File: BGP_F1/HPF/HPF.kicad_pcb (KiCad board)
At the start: 2 copper layers, 30 x 24 mm, 15 parts, among them P1 CONN_01X05, P2 CONN_01X06, U1 MC33178

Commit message: F1 updates to reverse pots
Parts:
- C3: value 39n -> 22n
- R3, R5, R7: value 4.99k -> 4.7k
- R4: value 24.9k -> 24k
- R6: value 49.9k -> 47k
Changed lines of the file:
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@@
       (effects (font (size 0.6 0.6) (thickness 0.15)))
     )
-    (fp_text value 39n (at 0 2.3 180) (layer F.Fab) hide
+    (fp_text value 22n (at 0 2.3 180) (layer F.Fab) hide
       (effects (font (size 0.6 0.6) (thickness 0.15)))
     )
@@
       (effects (font (size 0.6 0.6) (thickness 0.15)))
     )
-    (fp_text value 4.99k (at 0 1.9) (layer F.Fab) hide
+    (fp_text value 4.7k (at 0 1.9) (layer F.Fab) hide
       (effects (font (size 0.6 0.6) (thickness 0.15)))
     )
@@
       (effects (font (size 0.6 0.6) (thickness 0.15)))
     )
-    (fp_text value 24.9k (at 0 1.9 180) (layer F.Fab) hide
+    (fp_text value 24k (at 0 1.9 180) (layer F.Fab) hide
       (effects (font (size 0.6 0.6) (thickness 0.15)))
     )
@@
       (effects (font (size 0.6 0.6) (thickness 0.15)))
     )
-    (fp_text value 4.99k (at 0 1.9 180) (layer F.Fab) hide
+    (fp_text value 4.7k (at 0 1.9 180) (layer F.Fab) hide
       (effects (font (size 0.6 0.6) (thickness 0.15)))
     )
@@
       (effects (font (size 0.6 0.6) (thickness 0.15)))
     )
-    (fp_text value 49.9k (at 0 1.9) (layer F.Fab) hide
+    (fp_text value 47k (at 0 1.9) (layer F.Fab) hide
       (effects (font (size 0.6 0.6) (thickness 0.15)))
     )
@@
       (effects (font (size 0.6 0.6) (thickness 0.15)))
     )
-    (fp_text value 4.99k (at 0 1.9 270) (layer F.Fab) hide
-      (effects (font (size 0.6 0.6) (thickness 0.15)))
-    )
+    (fp_text value 4.7k (at 0 1.9 270) (layer F.Fab) hide
+      (effects (font (size 0.6 0.6) (thickness 0.15)))
+    )

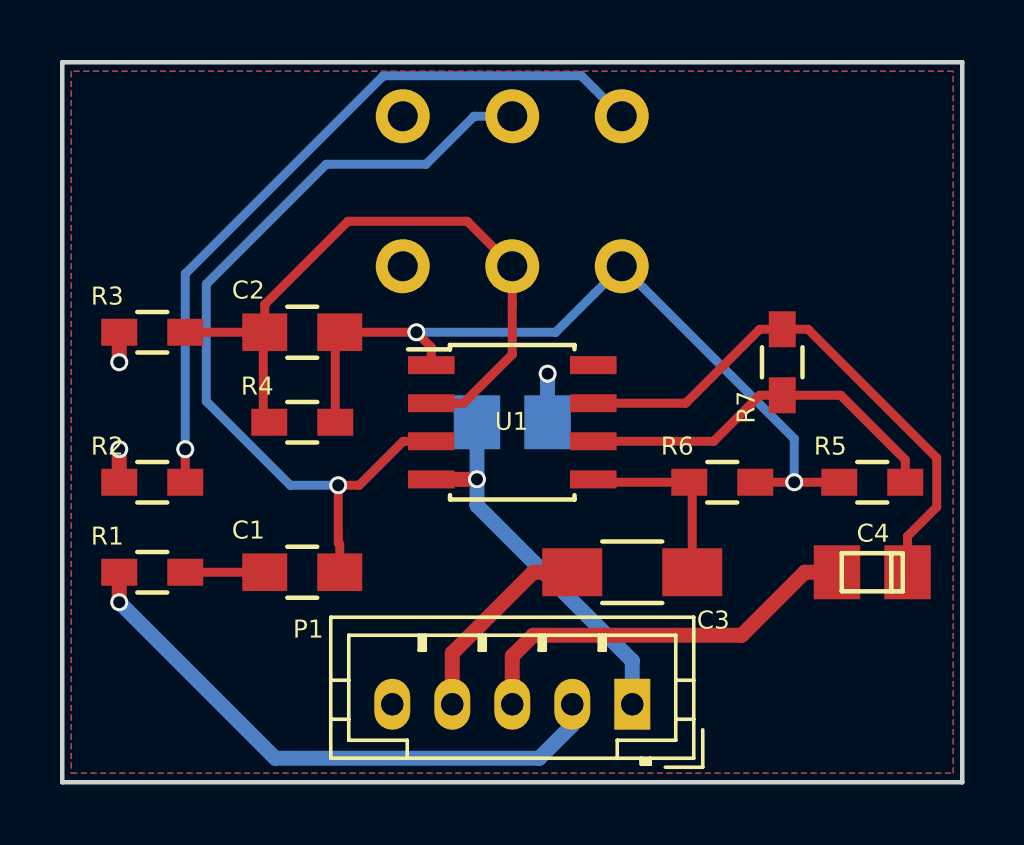
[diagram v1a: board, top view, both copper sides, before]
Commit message: HPF Done
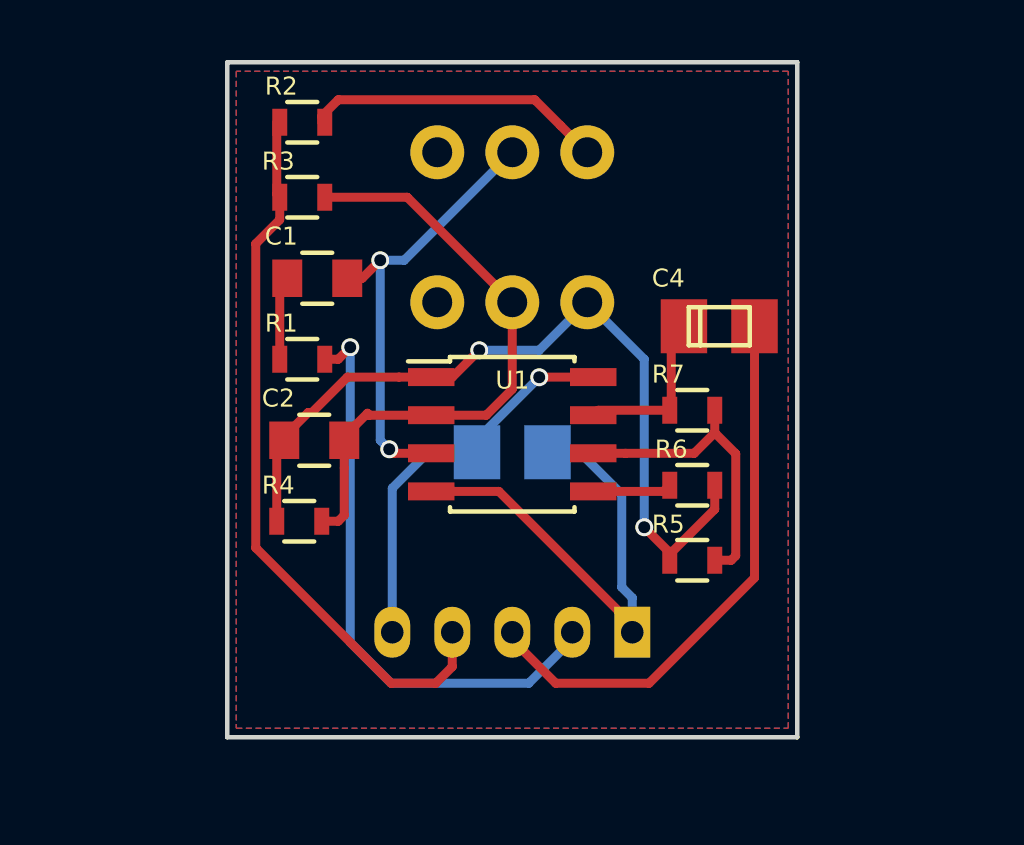
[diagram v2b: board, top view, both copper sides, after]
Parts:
- removed C3: 22n, Capacitors_SMD:C_1206_HandSoldering
- C1, C2: footprint Capacitors_SMD:C_0805_HandSoldering -> Capacitors_SMD:C_0805
- P1: moved to B.Cu
- P2: footprint LIBS:Potentiometer_Alpha_Double_Vertical_Dual_Shaft -> LIBS:Potentiometer_Alps_RK097_Double_Vertical_Dual_Shaft
- R1, R2, R3, R4, R5, R6, R7: footprint Resistors_SMD:R_0603_HandSoldering -> Resistors_SMD:R_0603
- moved R2 13.0 mm to (151.0, 89.0)
- moved C1 9.81 mm to (151.5, 94.2)
- moved C4 9.66 mm to (164.9, 95.8), turned to 180 degrees
- moved R1 8.68 mm to (151.0, 96.9), turned to 0 degrees
- moved R3 6.73 mm to (151.0, 91.5)
- moved R5 6.54 mm to (164.0, 103.6)
- moved C2 3.62 mm to (151.4, 99.6), turned to 0 degrees
- moved R7 3.40 mm to (164.0, 98.6), turned to 0 degrees
- moved R4 3.30 mm to (150.9, 102.3), turned to 0 degrees
- moved P1 2.40 mm to (162.0, 106.0)
- moved P2 1.66 mm to (155.5, 90.0)
- moved R6 1.00 mm to (164.0, 101.1)
- moved C5 1.00 mm to (158.0, 100.0), turned to 180 degrees
- moved U1 0.40 mm to (158.0, 99.4)
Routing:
- net /Vref: track 8.52 -> 24.4 mm, vias 2 -> 0
- net /VF_3: track 24.8 -> 10.0 mm, vias 1 -> 0
- net /VF_2: track 28.6 -> 15.1 mm, vias 1 -> 2
- net Net-(C4-Pad1): track 18.7 -> 5.61 mm
- net /V+: track 1.62 -> 13.3 mm
- net /OUT: track 13.2 -> 18.8 mm
- net Earth: track 12.7 -> 16.6 mm, vias 1 -> 0
- net Net-(C3-Pad1): track 6.28 -> 2.63 mm
- net /VG_2: track 23.0 -> 20.4 mm
- net Net-(R5-Pad1): track 12.7 -> 10.2 mm
- net /VG_3: track 27.3 -> 27.9 mm
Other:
- board size 30 x 24 mm -> 19 x 22.5 mm
